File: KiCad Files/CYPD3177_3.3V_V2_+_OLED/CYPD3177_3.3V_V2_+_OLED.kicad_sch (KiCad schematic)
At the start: 0 parts

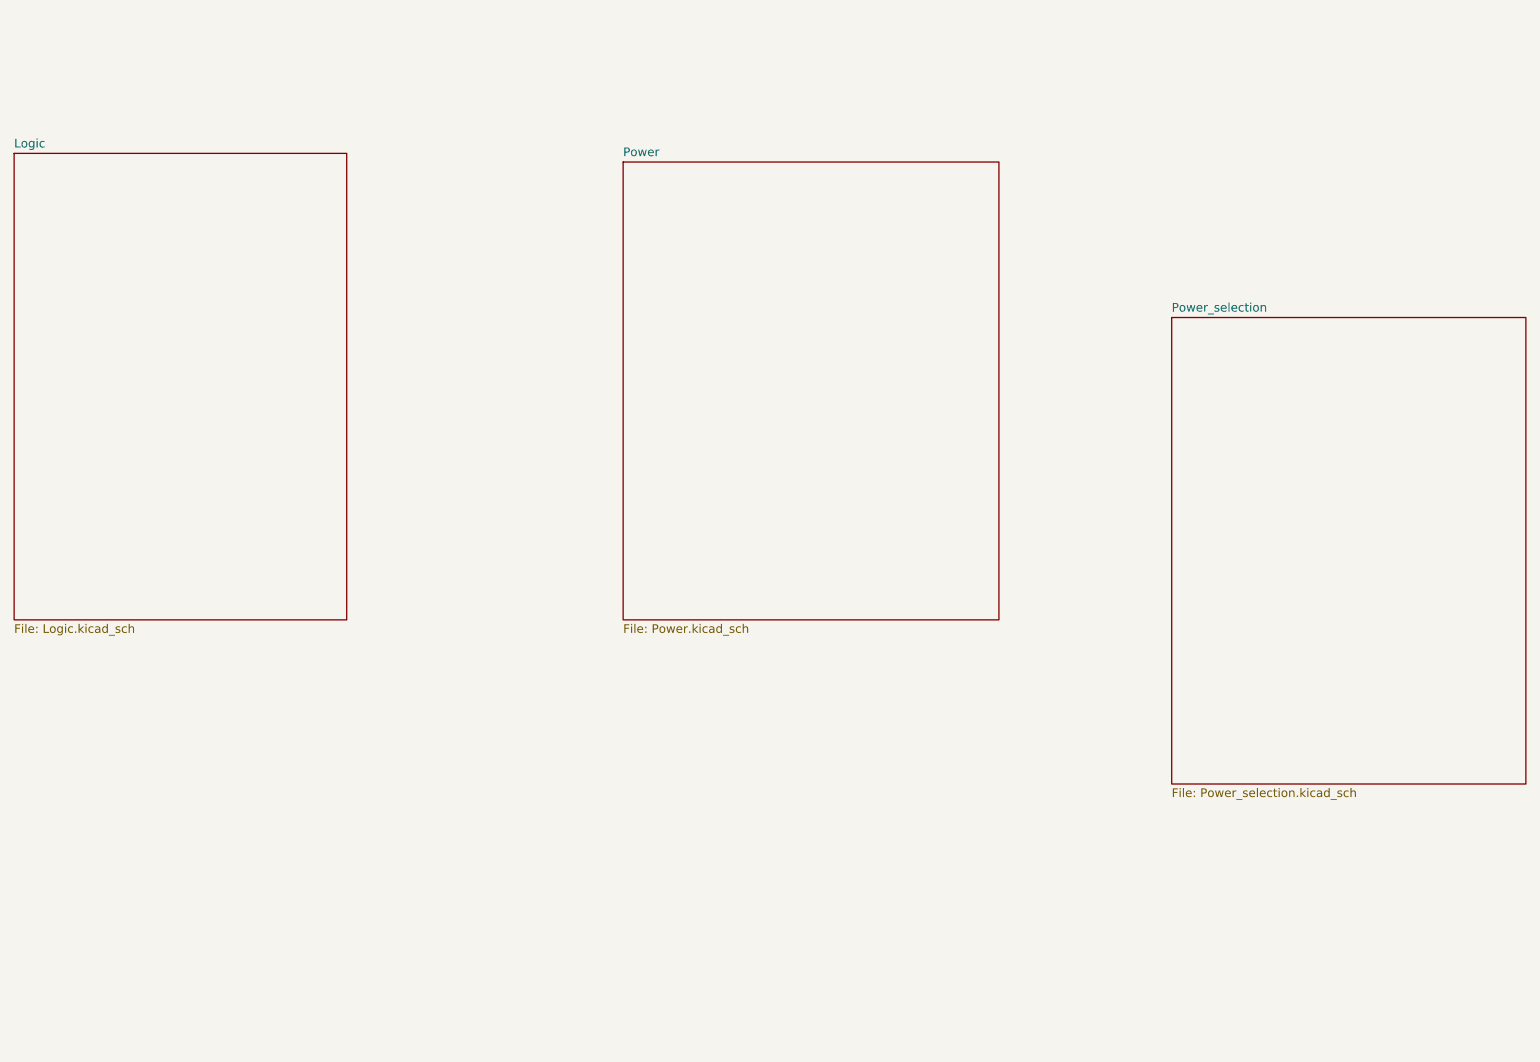
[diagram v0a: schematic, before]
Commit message: schematics done
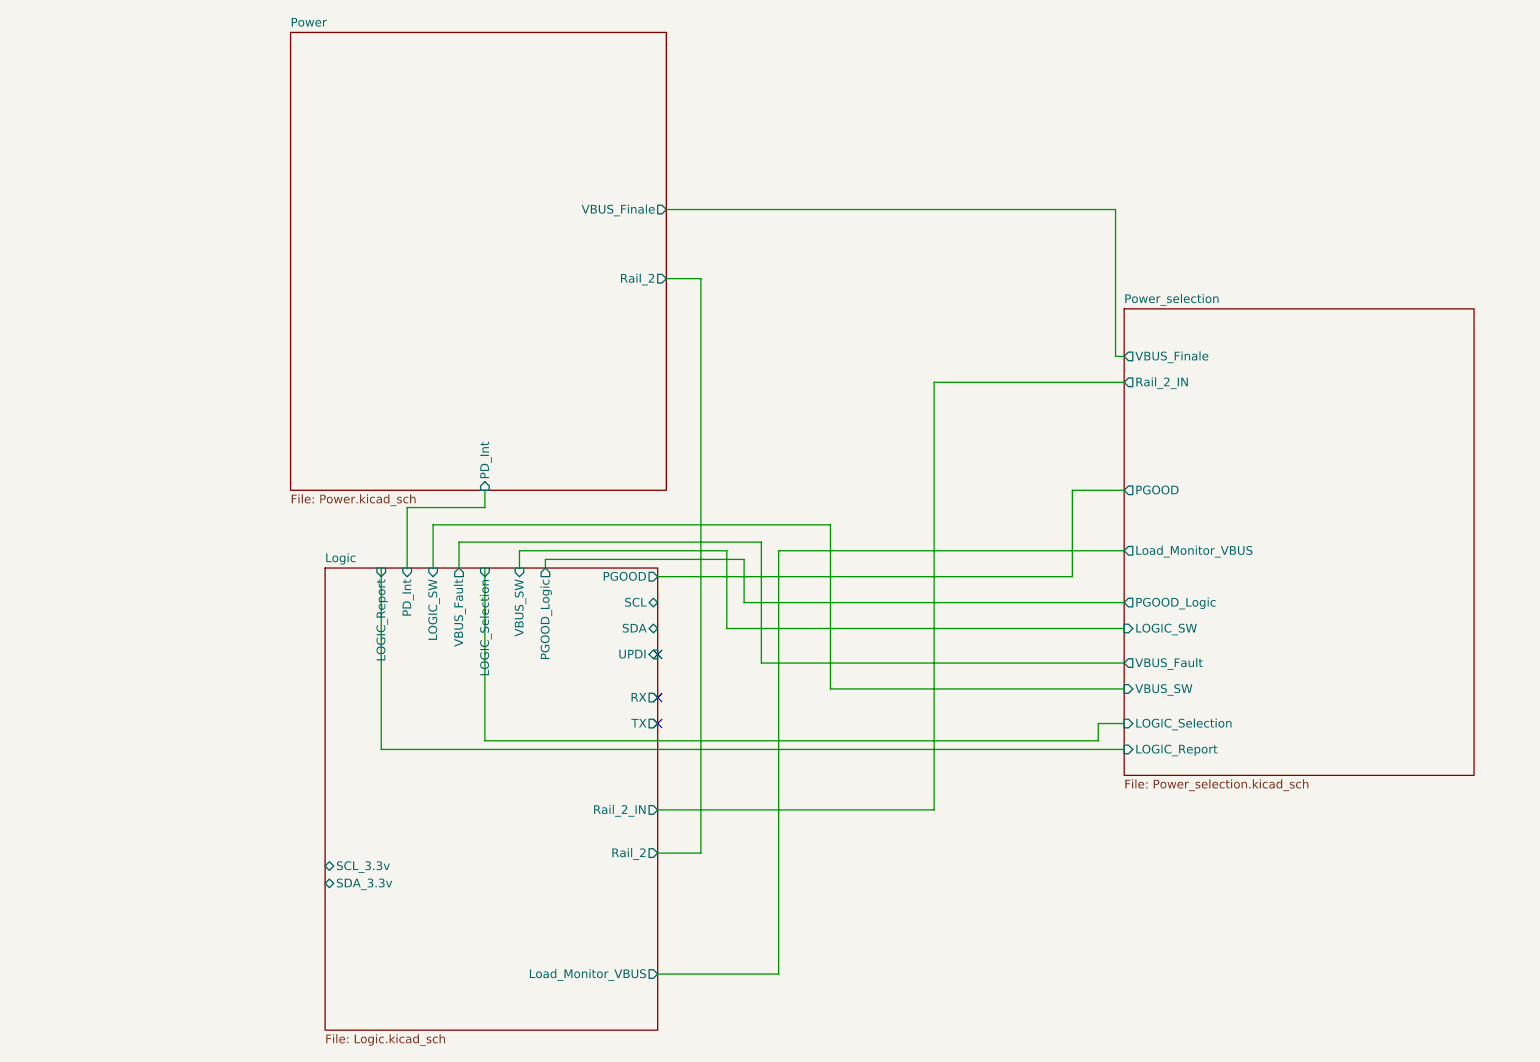
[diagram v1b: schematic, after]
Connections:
- no-connect marks 0 -> 3
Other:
- sheet Logic ports: added LOGIC_Report, LOGIC_SW, LOGIC_Selection, Load_Monitor_VBUS, PD_Int, PGOOD, PGOOD_Logic, RX, Rail_2, Rail_2_IN, SCL, SCL_3.3v, SDA, SDA_3.3v, TX, UPDI, VBUS_Fault, VBUS_SW; removed none
- sheet Power ports: added PD_Int, Rail_2, VBUS_Finale; removed none
- sheet Power_selection ports: added LOGIC_Report, LOGIC_SW, LOGIC_Selection, Load_Monitor_VBUS, PGOOD, PGOOD_Logic, Rail_2_IN, VBUS_Fault, VBUS_Finale, VBUS_SW; removed none
